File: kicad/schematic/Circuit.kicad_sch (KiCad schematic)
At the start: 81 parts, among them M1 Motor_DC, M2 Motor_DC, M3 Motor_DC, M4 Motor_DC, M5 Motor_DC, M6 Motor_DC, M7 Motor_DC, M8 Motor_DC, Q1 AO3400A, Q2 AO3400A, Q3 AO3400A, Q4 AO3400A, Q5 AO3400A, Q6 AO3400A, Q7 AO3400A, Q8 AO3400A, SW1 SW_Push

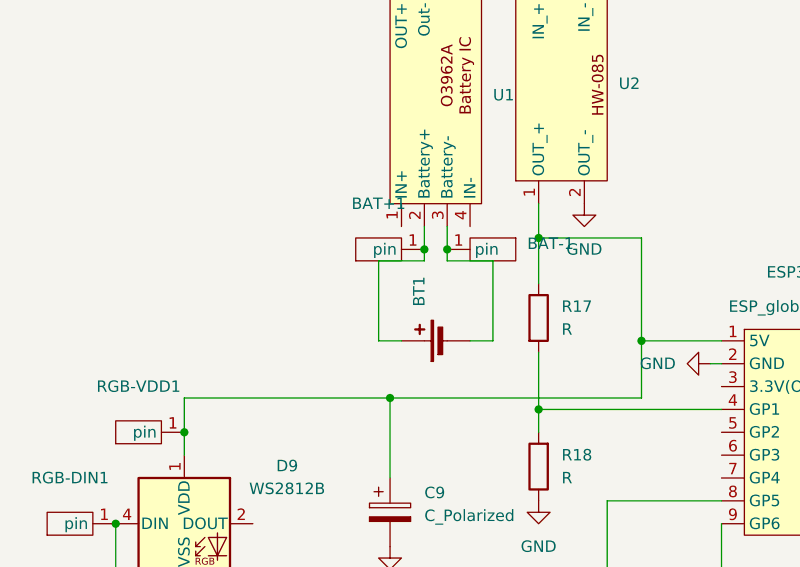
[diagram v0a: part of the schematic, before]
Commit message: almost final - text image missing
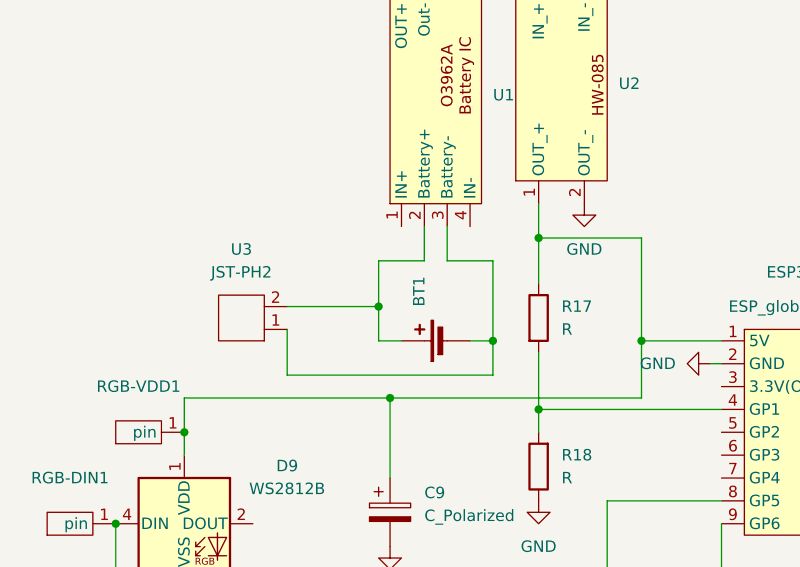
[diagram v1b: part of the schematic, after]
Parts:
- removed BAT+1, BAT-1: ~, ESP_global:blank pad, symbol waveshare_esp32_s3_mini_zero:blank_pad_1
- added U3: JST-PH2, Connector_JST:JST_EH_S2B-EH_1x02_P2.50mm_Horizontal, symbol SonicSensor:SensorConnecter
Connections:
- net at BT1.1 (+), U1.2 (Battery+): now also U3.2
- net at BT1.2 (-), U1.3 (Battery-): now also U3.1
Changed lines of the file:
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@@
 	(paper "A3")
 	(junction
-		(at 148.59 88.9)
-		(diameter 0)
-		(color 0 0 0 0)
-	)
-	(junction
 		(at 236.22 53.34)
 		(diameter 0)
@@
 	)
 	(junction
-		(at 146.05 88.9)
-		(diameter 0)
-		(color 0 0 0 0)
-	)
-	(junction
 		(at 269.24 106.68)
 		(diameter 0)
@@
 	)
 	(junction
+		(at 140.97 95.25)
+		(diameter 0)
+		(color 0 0 0 0)
+	)
+	(junction
 		(at 278.13 124.46)
 		(diameter 0)
@@
 	)
 	(junction
+		(at 153.67 99.06)
+		(diameter 0)
+		(color 0 0 0 0)
+	)
+	(junction
 		(at 278.13 101.6)
 		(diameter 0)
@@
 	(wire
 		(pts
+			(xy 153.67 102.87) (xy 130.81 102.87)
+		)
+		(stroke
+			(width 0)
+			(type default)
+		)
+	)
+	(wire
+		(pts
 			(xy 278.13 62.23) (xy 278.13 64.77)
 		)
@@
 	(wire
 		(pts
-			(xy 140.97 90.17) (xy 140.97 99.06)
+			(xy 140.97 90.17) (xy 140.97 95.25)
 		)
 		(stroke
@@
 	(wire
 		(pts
-			(xy 146.05 86.36) (xy 146.05 88.9)
-		)
-		(stroke
-			(width 0)
-			(type default)
-		)
-	)
-	(wire
-		(pts
 			(xy 269.24 160.02) (xy 269.24 162.56)
 		)
@@
 	(wire
 		(pts
+			(xy 153.67 99.06) (xy 153.67 102.87)
+		)
+		(stroke
+			(width 0)
+			(type default)
+		)
+	)
+	(wire
+		(pts
 			(xy 204.47 111.76) (xy 224.79 111.76)
 		)
@@
 	(wire
 		(pts
-			(xy 148.59 88.9) (xy 148.59 90.17)
-		)
-		(stroke
-			(width 0)
-			(type default)
-		)
-	)
-	(wire
-		(pts
 			(xy 119.38 105.41) (xy 119.38 109.22)
 		)
@@
 	(wire
 		(pts
+			(xy 140.97 95.25) (xy 140.97 99.06)
+		)
+		(stroke
+			(width 0)
+			(type default)
+		)
+	)
+	(wire
+		(pts
 			(xy 179.07 119.38) (xy 179.07 182.88)
 		)
@@
 	(wire
 		(pts
-			(xy 146.05 88.9) (xy 146.05 90.17)
+			(xy 146.05 86.36) (xy 146.05 90.17)
 		)
 		(stroke
@@
 	(wire
 		(pts
-			(xy 148.59 86.36) (xy 148.59 88.9)
+			(xy 148.59 86.36) (xy 148.59 90.17)
 		)
 		(stroke
@@
 	(wire
 		(pts
+			(xy 130.81 95.25) (xy 140.97 95.25)
+		)
+		(stroke
+			(width 0)
+			(type default)
+		)
+	)
+	(wire
+		(pts
 			(xy 269.24 124.46) (xy 265.43 124.46)
 		)
@@
 	(wire
 		(pts
+			(xy 130.81 97.79) (xy 130.81 102.87)
+		)
+		(stroke
+			(width 0)
+			(type default)
+		)
+	)
+	(wire
+		(pts
 			(xy 289.56 106.68) (xy 278.13 106.68)
 		)
@@
 	)
 	(symbol
-		(lib_id "waveshare_esp32_s3_mini_zero:blank_pad_1")
-		(at 153.67 88.9 270)
-		(unit 1)
-		(exclude_from_sim no)
-		(in_bom yes)
-		(on_board yes)
-		(dnp no)
-		(fields_autoplaced yes)
-		(property "Reference" "BAT-1"
-			(at 157.48 88.2649 90)
-			(effects
-				(font
-					(size 1.27 1.27)
-				)
-				(justify left)
-			)
-		)
-		(property "Value" "~"
-			(at 157.48 90.17 90)
-			(effects
-				(font
-					(size 1.27 1.27)
-				)
-				(justify left)
-			)
-		)
-		(property "Footprint" "ESP_global:blank pad"
-			(at 153.67 88.9 0)
-			(effects
-				(font
-					(size 1.27 1.27)
-				)
-				(hide yes)
-			)
-		)
-		(property "Datasheet" ""
-			(at 153.67 88.9 0)
-			(effects
-				(font
-					(size 1.27 1.27)
-				)
-				(hide yes)
-			)
-		)
-		(property "Description" ""
-			(at 153.67 88.9 0)
-			(effects
-				(font
-					(size 1.27 1.27)
-				)
-				(hide yes)
-			)
-		)
-		(pin "1"
-		)
-		(instances
-			(project "Circuit"
-				(path "/b1011026-c160-485a-bf1a-9bf26ac94018"
-					(reference "BAT-1")
-					(unit 1)
-				)
-			)
-		)
-	)
-	(symbol
 		(lib_id "Device:C")
 		(at 269.24 130.81 180)
@@
 	)
 	(symbol
+		(lib_id "SonicSensor:SensorConnecter")
+		(at 125.73 96.52 180)
+		(unit 1)
+		(exclude_from_sim no)
+		(in_bom yes)
+		(on_board yes)
+		(dnp no)
+		(fields_autoplaced yes)
+		(property "Reference" "U3"
+			(at 125.73 88.9 0)
+			(effects
+				(font
+					(size 1.27 1.27)
+				)
+			)
+		)
+		(property "Value" "JST-PH2"
+			(at 125.73 91.44 0)
+			(effects
+				(font
+					(size 1.27 1.27)
+				)
+			)
+		)
+		(property "Footprint" "Connector_JST:JST_EH_S2B-EH_1x02_P2.50mm_Horizontal"
+			(at 125.73 96.52 0)
+			(effects
+				(font
+					(size 1.27 1.27)
+				)
+				(hide yes)
+			)
+		)
+		(property "Datasheet" ""
+			(at 125.73 96.52 0)
+			(effects
+				(font
+					(size 1.27 1.27)
+				)
+				(hide yes)
+			)
+		)
+		(property "Description" ""
+			(at 125.73 96.52 0)
+			(effects
+				(font
+					(size 1.27 1.27)
+				)
+				(hide yes)
+			)
+		)
+		(pin "2"
+		)
+		(pin "1"
+		)
+		(instances
+			(project ""
+				(path "/b1011026-c160-485a-bf1a-9bf26ac94018"
+					(reference "U3")
+					(unit 1)
+				)
+			)
+		)
+	)
+	(symbol
 		(lib_id "power:GND")
 		(at 142.24 121.92 0)
@@
 					(unit 1)
 				)
-			)
-		)
-	)
-	(symbol
-		(lib_id "waveshare_esp32_s3_mini_zero:blank_pad_1")
-		(at 140.97 88.9 90)
-		(unit 1)
-		(exclude_from_sim no)
-		(in_bom yes)
-		(on_board yes)
-		(dnp no)
-		(fields_autoplaced yes)
-		(property "Reference" "BAT+1"
-			(at 140.97 83.82 90)
-			(effects
-				(font
-					(size 1.27 1.27)
-				)
-			)
-		)
-		(property "Value" "~"
-			(at 140.97 86.36 90)
-			(effects
-				(font
-					(size 1.27 1.27)
-				)
-			)
-		)
-		(property "Footprint" "ESP_global:blank pad"
-			(at 140.97 88.9 0)
-			(effects
-				(font
-					(size 1.27 1.27)
-				)
-				(hide yes)
-			)
-		)
-		(property "Datasheet" ""
-			(at 140.97 88.9 0)
-			(effects
-				(font
-					(size 1.27 1.27)
-				)
-				(hide yes)
-			)
-		)
-		(property "Description" ""
-			(at 140.97 88.9 0)
-			(effects
-				(font
-					(size 1.27 1.27)
-				)
-				(hide yes)
-			)
-		)
-		(pin "1"
-		)
-		(instances
-			(project "Circuit"
-				(path "/b1011026-c160-485a-bf1a-9bf26ac94018"
-					(reference "BAT+1")
-					(unit 1)
-				)
